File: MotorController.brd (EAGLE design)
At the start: 100.4 x 41.1 mm, 13 parts

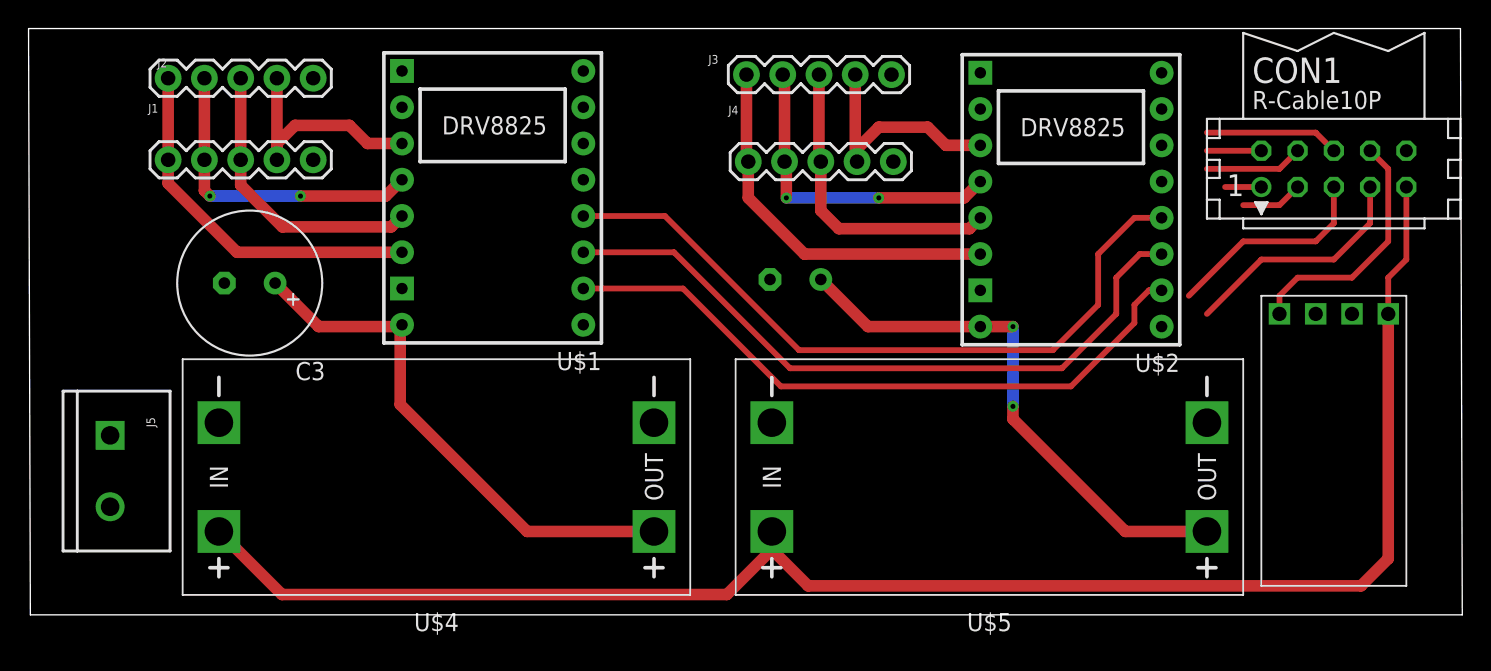
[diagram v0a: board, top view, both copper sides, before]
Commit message: pcb design waiting for inspection
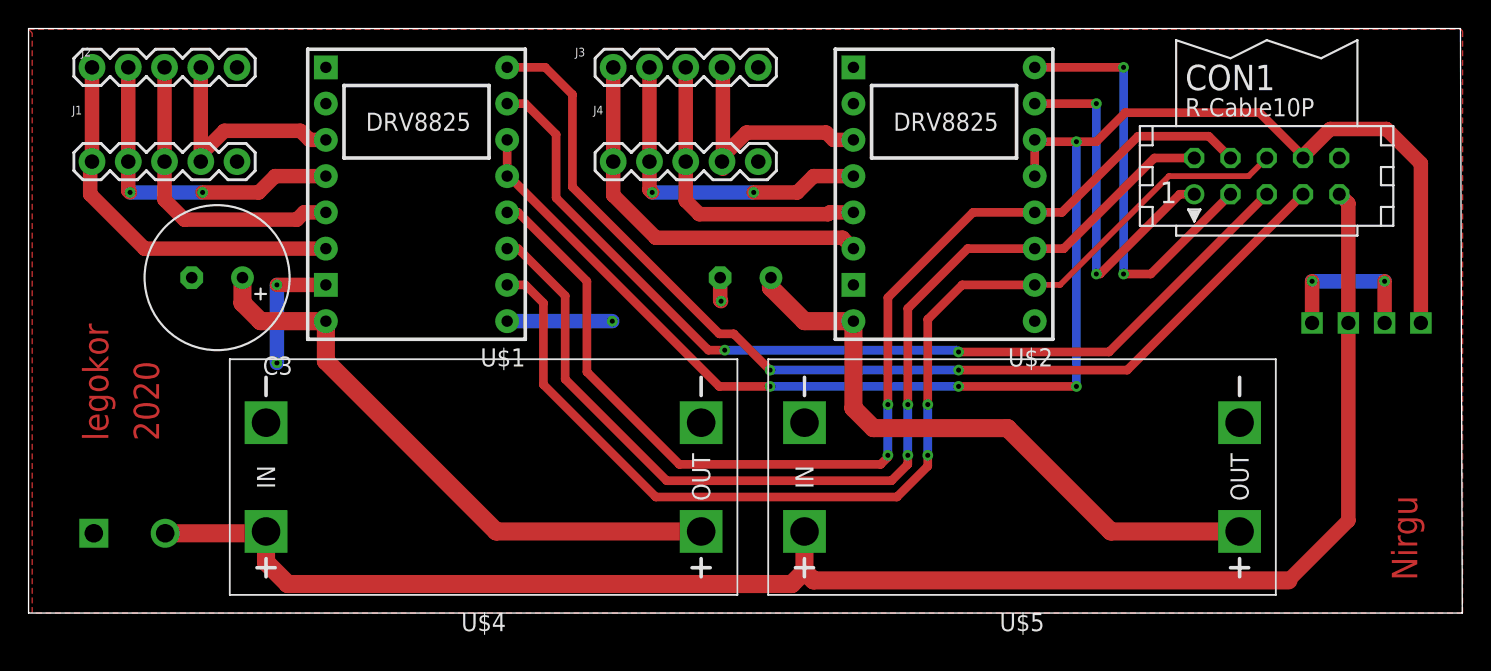
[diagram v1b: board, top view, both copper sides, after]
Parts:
- moved J4 9.46 mm to (41.0, 31.0)
- moved J3 9.35 mm to (41.0, 37.6)
- moved U$2 8.90 mm to (64.1, 28.7)
- moved J5 6.95 mm to (4.57, 4.95), flipped to the bottom, turned to 180 degrees
- moved J2 5.39 mm to (4.45, 37.6)
- moved U$1 5.34 mm to (27.2, 28.7)
- moved J1 5.34 mm to (4.45, 31.0)
- moved CON1 4.73 mm to (86.7, 30.0)
- moved C2 3.49 mm to (50.2, 22.9)
- moved U$4 3.30 mm to (31.9, 8.89)
- moved U$6 2.37 mm to (93.7, 19.7), flipped to the bottom
- moved C3 2.32 mm to (13.2, 22.9)
- moved U$5 2.29 mm to (69.6, 8.89)
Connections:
- removed net 5V: CON1.8, U$6.P$4
- removed net N$14: U$2.EN_N
- removed net N$9: U$1.EN_N
- net GND: now also U$1.EN_N, U$2.EN_N, U$6.P$3
- net VBAT: now also U$6.P$1; no longer U$6.P$3
- net VCC: now also CON1.8, U$6.P$4
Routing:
- net VCC: track 0.00 -> 110.5 mm, vias 0 -> 4
- net M_DIR2: track 16.6 -> 73.4 mm, vias 0 -> 2
- net M_STEP2: track 14.8 -> 67.6 mm, vias 0 -> 2
- net GND: track 0.00 -> 28.9 mm, vias 0 -> 6
- net M_DIR1: track 4.34 -> 30.5 mm, vias 0 -> 2
- net M_STEP1: track 2.54 -> 25.4 mm, vias 0 -> 2
- net M_M0: track 56.3 -> 78.6 mm, vias 0 -> 2
- net M_M1: track 52.5 -> 74.1 mm, vias 0 -> 2
- net M_M2: track 57.2 -> 78.4 mm, vias 0 -> 2
- net 5V: track 17.3 -> 0.00 mm
- net VMOT2: track 38.2 -> 44.2 mm, vias 2 -> 0
- net VMOT1: track 37.1 -> 42.2 mm
- net SIDEA_B2: track 25.7 -> 27.0 mm
- net SIDEA_B1: track 20.3 -> 21.4 mm
- net SIDEB_B2: track 26.6 -> 27.3 mm
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- added copper zone on layer 1, net GND
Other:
- board size 100.4 x 41.1 mm -> 100.4 x 40.9 mm
- board text added: "2020"
- board text added: "Nirgu"
- board text added: "legokor"
